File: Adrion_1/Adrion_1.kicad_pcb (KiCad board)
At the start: 4 copper layers, 193.4 x 230.1 mm, 112 parts, among them IC1 REF1933AIDDCR, IC2 UCC21521DW, IC3 UCC21521DW, J1 1705469, J2 1705469, J3 1729128, J6 M20-7821546, J7 M20-7821546, Q1 IPP111N15N3GXKSA1, Q2 IPP111N15N3GXKSA1, Q3 IPP111N15N3GXKSA1, Q5 IPP111N15N3GXKSA1, U3 NUCLEO-G431KB, U4 TPS7A2033PDBVR, U5 CKSR_6-NP

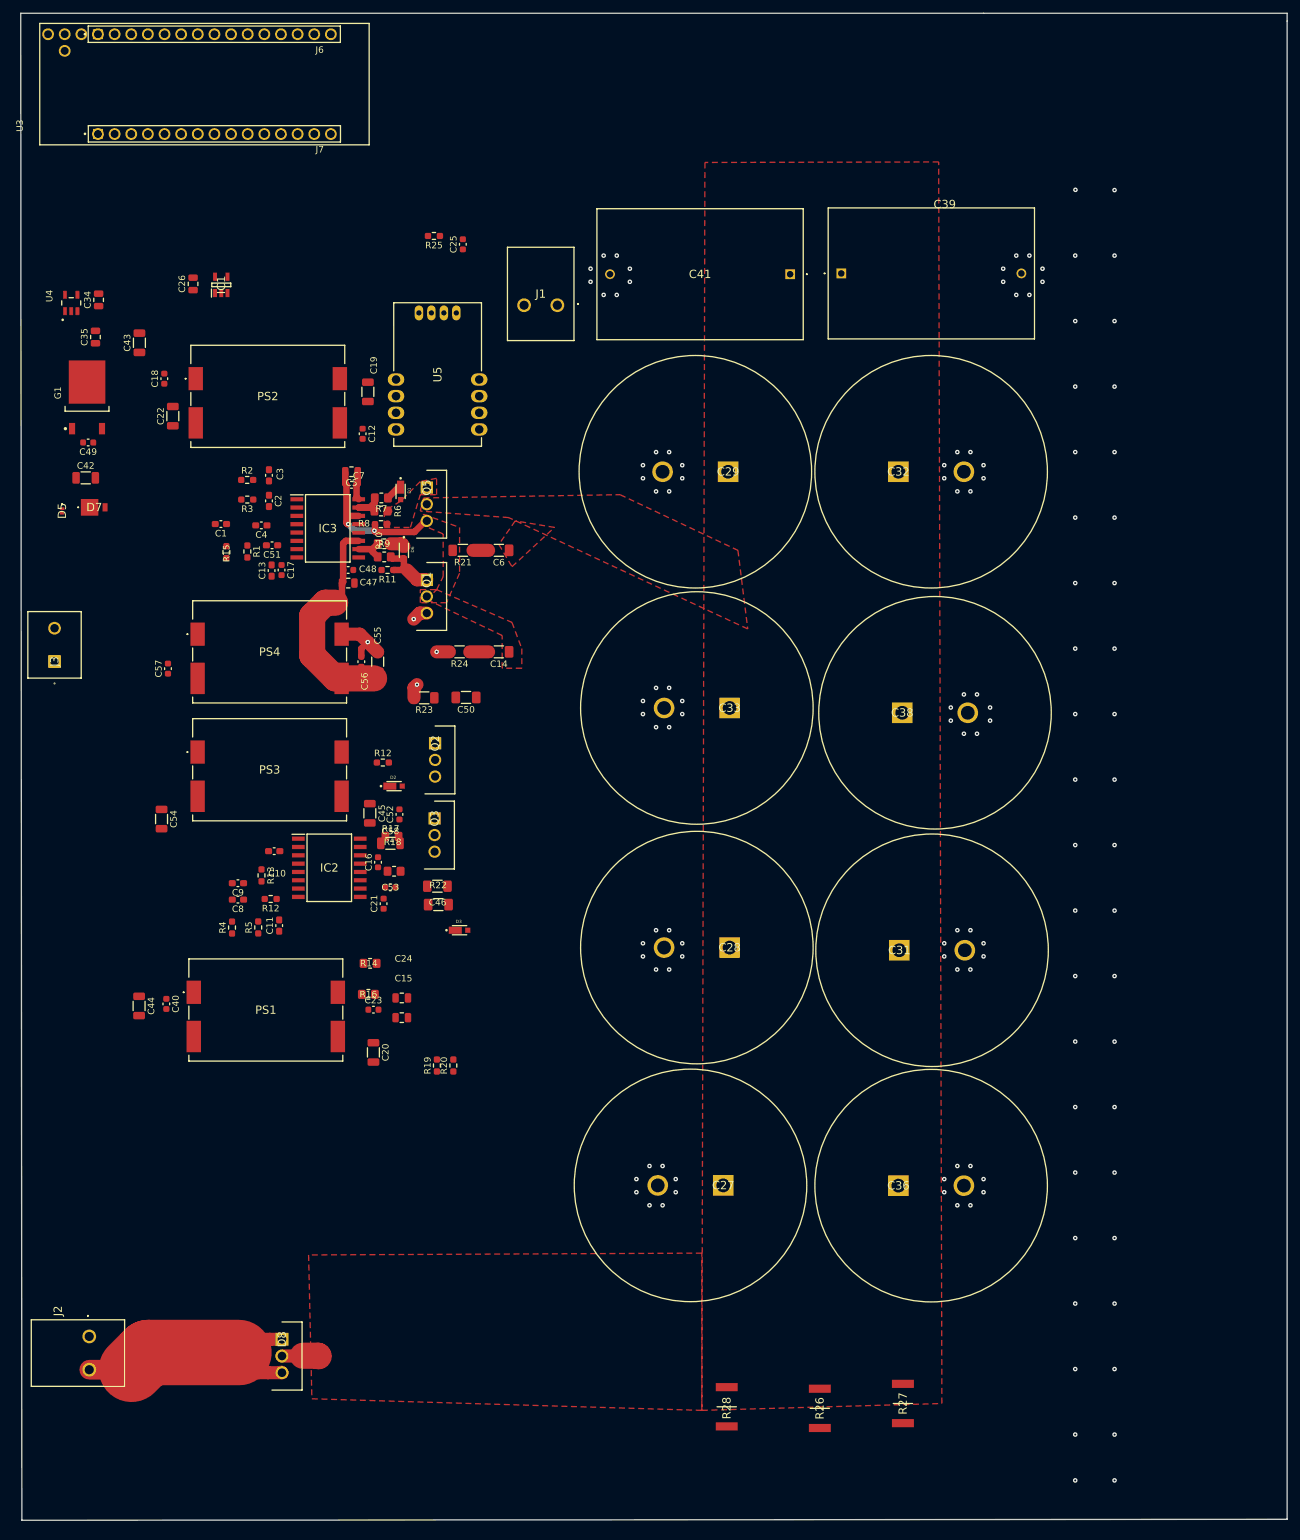
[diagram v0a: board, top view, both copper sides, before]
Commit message: Layout
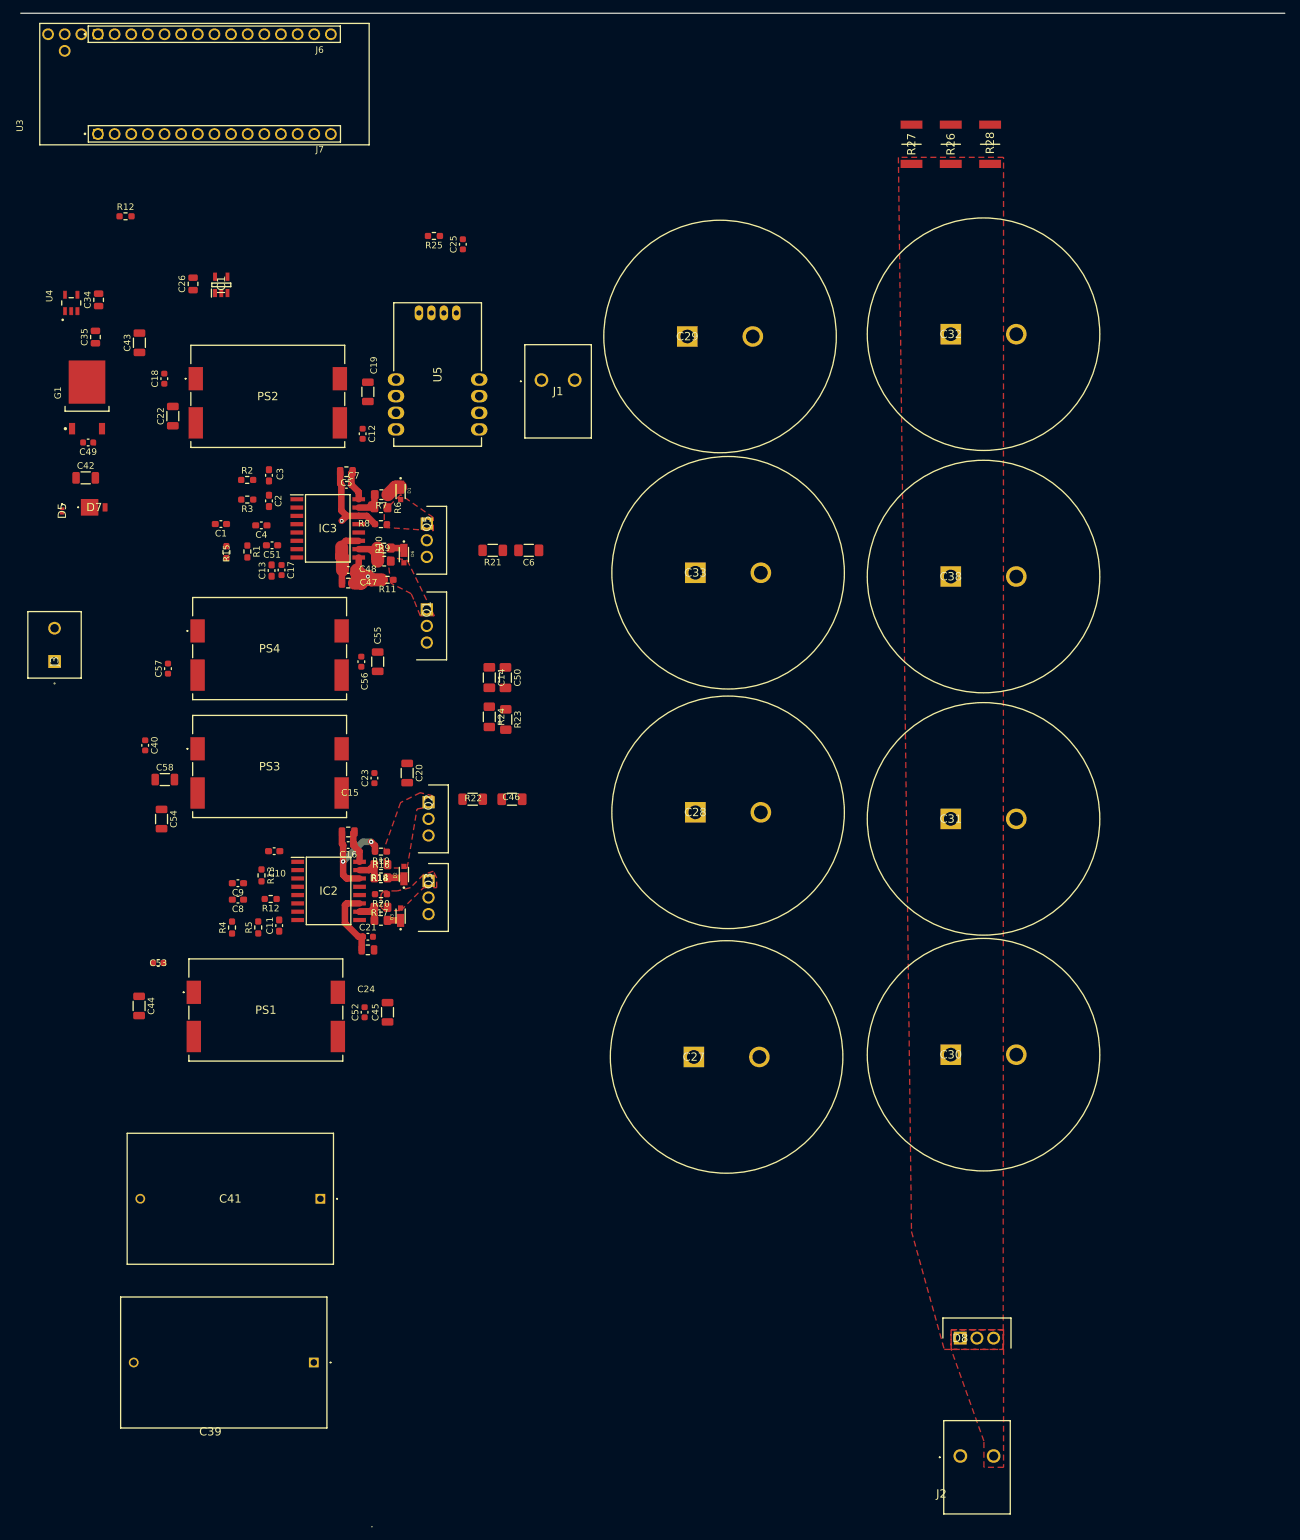
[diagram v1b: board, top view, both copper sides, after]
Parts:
- removed C36: B43547F2108M067, CAPPRD1000W190D3550H4200:CAPPRD1000W190D3550H4200
- added C30: B43547F2108M067, CAPPRD1000W190D3550H4200:CAPPRD1000W190D3550H4200, F.Cu at (155.0, 172.0)
- moved R28 196.9 mm to (161.0, 33.0), turned to -90 degrees
- moved R26 194.0 mm to (155.0, 33.0), turned to -90 degrees
- moved R27 192.3 mm to (149.0, 33.0), turned to -90 degrees
- moved C39 184.8 mm to (57.8, 219.0), turned to 180 degrees
- moved C41 158.3 mm to (58.8, 194.0)
- moved J2 134.2 mm to (156.5, 233.3), turned to 0 degrees
- moved D8 103.6 mm to (156.4, 215.3), turned to 0 degrees
- moved R12 92.2 mm to (29.0, 44.0)
- moved C20 43.0 mm to (72.0, 129.0)
- moved C40 39.6 mm to (32.0, 124.8)
- moved C53 37.3 mm to (34.0, 158.0)
- moved C58 35.8 mm to (35.0, 130.0)
- moved C23 35.4 mm to (67.0, 129.8), turned to 90 degrees
- moved R19 33.8 mm to (68.0, 141.0), turned to 180 degrees
- moved C52 30.7 mm to (65.5, 165.5)
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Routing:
- net Net-(D8-Pad1): track 31.8 -> 0.00 mm
- net Net-(IC3-VDDB): track 33.3 -> 8.81 mm
- net Net-(IC2-VSSA): track 0.00 -> 16.6 mm, vias 0 -> 2
- net Net-(IC3-VSSA): track 25.3 -> 13.1 mm, vias 2 -> 1
- net Net-(IC2-VDDB): track 0.00 -> 10.8 mm
- net Net-(Q1-G): track 9.77 -> 0.00 mm
- net Net-(IC2-OUTB): track 0.00 -> 5.98 mm
- net HV: track 5.65 -> 0.00 mm
- net Net-(IC2-VDDA): track 0.00 -> 5.27 mm
- net GNDPWR: track 15.8 -> 10.7 mm, vias 126 -> 1
- net Net-(IC2-OUTA): track 0.00 -> 4.62 mm
- net Net-(C14-Pad2): track 2.89 -> 0.00 mm
- net Net-(D2-Pad1): track 0.00 -> 2.56 mm
- net Net-(C6-Pad2): track 2.39 -> 0.00 mm
- net Net-(D3-Pad1): track 0.00 -> 2.00 mm
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- added copper zone on In2.Cu, net HV
- added copper zone on F.Cu, net Net-(D8-Pad1)
- added copper zone on F.Cu, net Net-(Q1-G)
- added copper zone on F.Cu, net Net-(Q2-G)
- added copper zone on F.Cu, net Net-(Q3-G)
- removed copper zone on F.Cu, net Net-(IC3-VSSA)
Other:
- board size 193.4 x 230.1 mm -> 193 x 231.1 mm
